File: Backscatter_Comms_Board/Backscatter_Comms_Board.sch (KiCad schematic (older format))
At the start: 49 parts, among them J1 SPK_IN, J2 Conn_01x11, J3 Conn_Coaxial_Power, M1 3SK293, T1 SP-48, U1 ADG919BRMZ, U2 ADG841YKSZ-REEL7, U3 NCS2200SQ2T2G

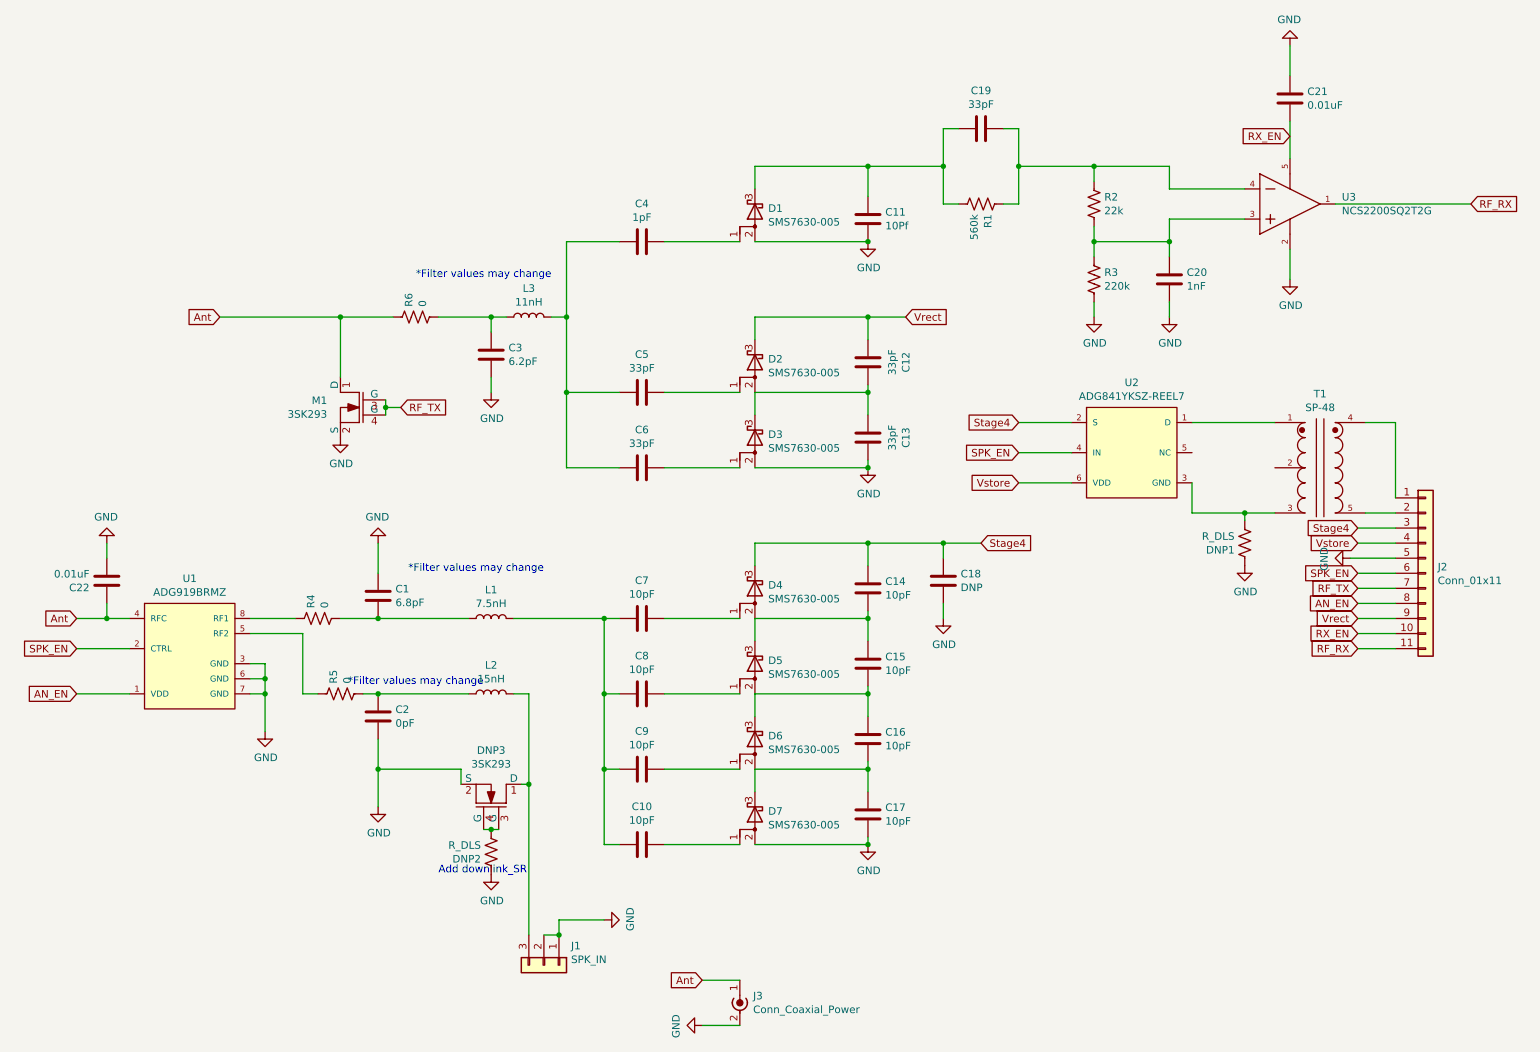
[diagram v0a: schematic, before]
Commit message: trying to make commit workj >:(
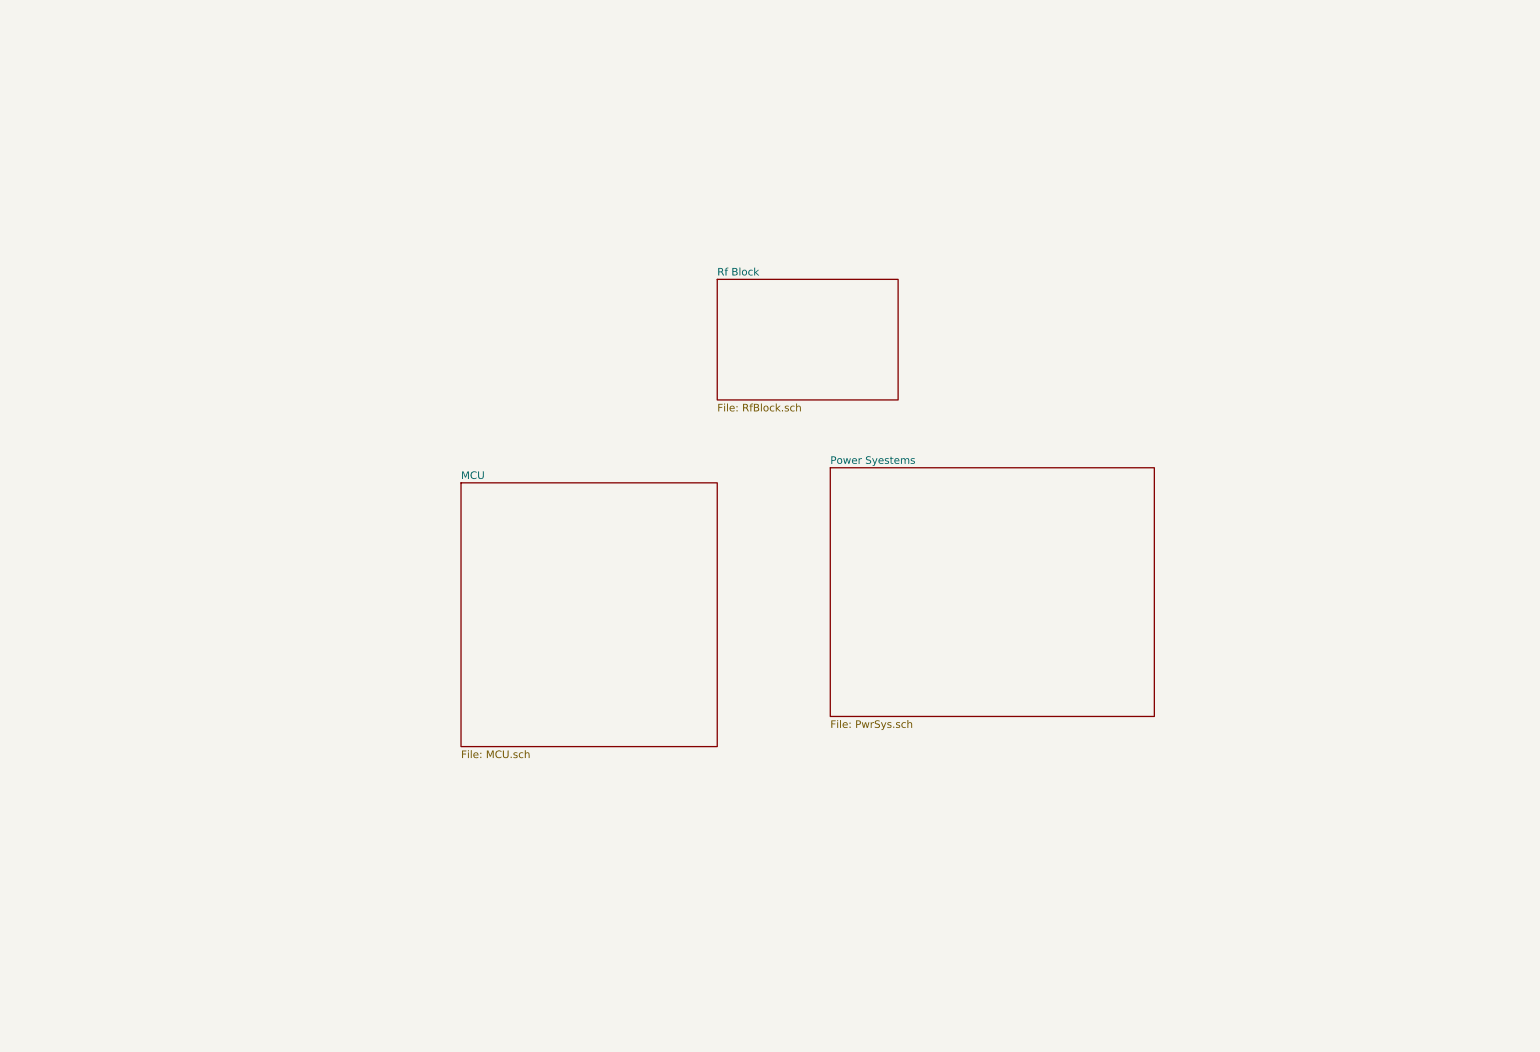
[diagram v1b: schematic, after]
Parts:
- removed C1: 6.8pF, Capacitor_SMD:C_0402_1005Metric_Pad0.74x0.62mm_HandSolder, symbol Device:C
- removed C10, C14, C15, C16, C17, C7, C8, C9: 10pF, Capacitor_SMD:C_0402_1005Metric_Pad0.74x0.62mm_HandSolder, symbol Device:C
- removed C11: 10Pf, Capacitor_SMD:C_0402_1005Metric_Pad0.74x0.62mm_HandSolder, symbol Device:C
- removed C12, C13, C19, C5, C6: 33pF, Capacitor_SMD:C_0402_1005Metric_Pad0.74x0.62mm_HandSolder, symbol Device:C
- removed C18: DNP, Capacitor_SMD:C_0402_1005Metric_Pad0.74x0.62mm_HandSolder, symbol Device:C
- removed C2: 0pF, Capacitor_SMD:C_0402_1005Metric_Pad0.74x0.62mm_HandSolder, symbol Device:C
- removed C20: 1nF, Capacitor_SMD:C_0402_1005Metric_Pad0.74x0.62mm_HandSolder, symbol Device:C
- removed C21, C22: 0.01uF, Capacitor_SMD:C_0402_1005Metric_Pad0.74x0.62mm_HandSolder, symbol Device:C
- removed C3: 6.2pF, Capacitor_SMD:C_0402_1005Metric_Pad0.74x0.62mm_HandSolder, symbol Device:C
- removed C4: 1pF, Capacitor_SMD:C_0402_1005Metric_Pad0.74x0.62mm_HandSolder, symbol Device:C
- removed D1, D2, D3, D4, D5, D6, D7: SMS7630-005, Local Components:SOT95P237X112-3N, symbol Device:D_Schottky_AAK
- removed DNP1, DNP2: R_DLS, Resistor_SMD:R_0402_1005Metric_Pad0.72x0.64mm_HandSolder, symbol Device:R_US
- removed DNP3, M1: 3SK293, Local Components:3SK293, symbol ADG919:3SK293
- removed J1: SPK_IN, Local Components:Multi-purpose_mic, symbol Connector_Generic:Conn_01x03
- removed J2: Conn_01x11, Connector_PinHeader_2.54mm:PinHeader_1x11_P2.54mm_Vertical, symbol Connector_Generic:Conn_01x11
- removed J3: Conn_Coaxial_Power, Connector_Coaxial:MMCX_Molex_73415-0961_Horizontal_0.8mm-PCB, symbol Connector:Conn_Coaxial_Power
- removed L1: 7.5nH, Inductor_SMD:L_0402_1005Metric, symbol Device:L
- removed L2: 15nH, Inductor_SMD:L_0402_1005Metric, symbol Device:L
- removed L3: 11nH, Inductor_SMD:L_0402_1005Metric, symbol Device:L
- removed R1: 560k, Resistor_SMD:R_0402_1005Metric_Pad0.72x0.64mm_HandSolder, symbol Device:R_US
- removed R2: 22k, Resistor_SMD:R_0402_1005Metric_Pad0.72x0.64mm_HandSolder, symbol Device:R_US
- removed R3: 220k, Resistor_SMD:R_0402_1005Metric_Pad0.72x0.64mm_HandSolder, symbol Device:R_US
- removed R4, R5, R6: 0, Resistor_SMD:R_0402_1005Metric_Pad0.72x0.64mm_HandSolder, symbol Device:R_US
- removed T1: SP-48, Local Components:XFMR_SP-48, symbol SP-48:SP-48
- removed U1: ADG919BRMZ, Local Components:Analog_Devices-ADG919BRMZ-Level_C, symbol ADG919:ADG919BRMZ
- removed U2: ADG841YKSZ-REEL7, Local Components:Analog_Devices-ADG841YKSZ-REEL7-Level_C, symbol ADG841:ADG841YKSZ-REEL7
- removed U3: NCS2200SQ2T2G, Local Components:On_Semiconductor-NCS2200SQ2T2G-Manufacturer_Recommended, symbol A_Comparator:NCS2200SQ2T2G
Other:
- note removed: "*Filter values may change\n"
- note removed: "Add downlink_SR\n"
